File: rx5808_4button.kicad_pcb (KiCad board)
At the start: 2 copper layers, 80 x 65 mm, 59 parts, among them IC1 ATMEGA328-A, P1 CONN_01X02, P10 CONN_01X01, P11 CONN_01X01, P2 CONN_01X05, P3 CONN_02X03, P5 BNC, P6 BNC, P7 CONN_01X02, P8 CONN_01X01, P9 CONN_01X01, SW1 SWITCH_INV, U1 TPS62160, U2 RX5808, U3 RF15-Punktlicht, U4 RF15-Punktlicht, U5 RF15-Punktlicht, U6 RF15-Punktlicht, Y1 16 MHz

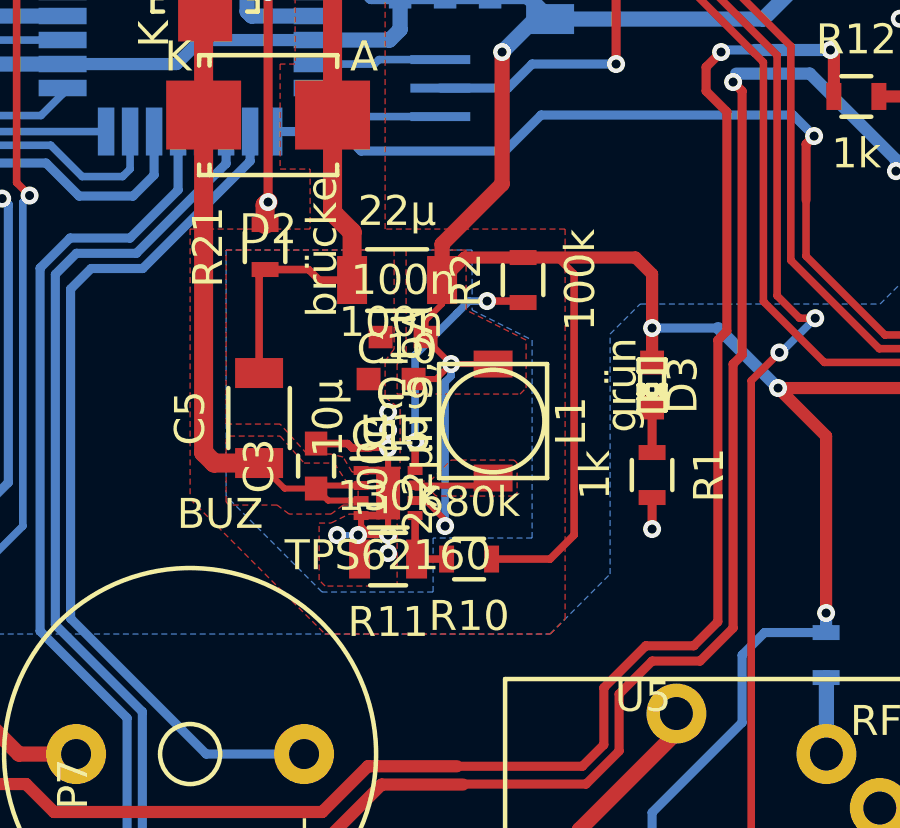
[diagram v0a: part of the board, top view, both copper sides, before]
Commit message: Schaltwandler weiter verbessert
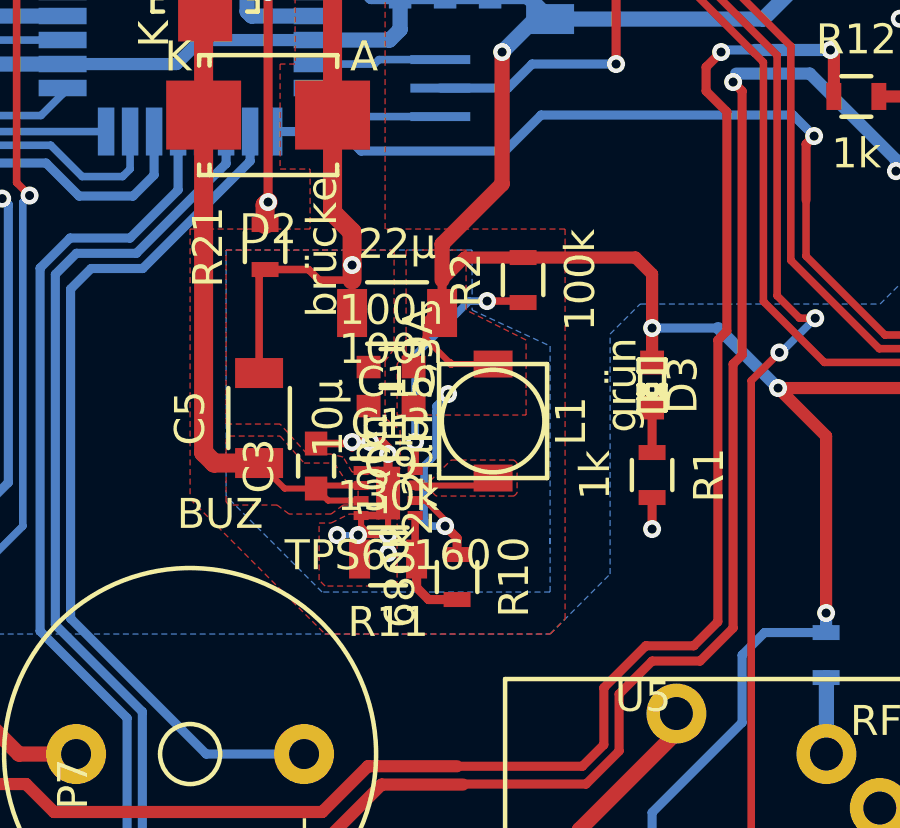
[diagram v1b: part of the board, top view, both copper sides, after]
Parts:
- moved C9 2.33 mm to (105.7, 96.4)
- moved C10 1.10 mm to (105.9, 93.3)
- moved R10 0.72 mm to (107.9, 102.1), turned to 270 degrees
- moved C13 0.40 mm to (105.7, 95.1)
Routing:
- net +5V: track 242.9 -> 229.9 mm
- net Net-(R10-Pad2): track 2.47 -> 3.94 mm
- net GNDPWR: track 36.3 -> 35.0 mm, vias 7 -> 8
